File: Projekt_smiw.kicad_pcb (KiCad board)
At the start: 4 copper layers, 66.9 x 38.2 mm, 24 parts, among them J1 USB_C_Receptacle_USB2.0, J4 Conn_02x12_Odd_Even, J5 Conn_02x12_Odd_Even, SW1 SW_Omron_B3FS, SW2 SW_Omron_B3FS, U1 USBLC6-2P6, U2 NCP1117-3.3_SOT223, U4 ESP32-S3-PICO-1

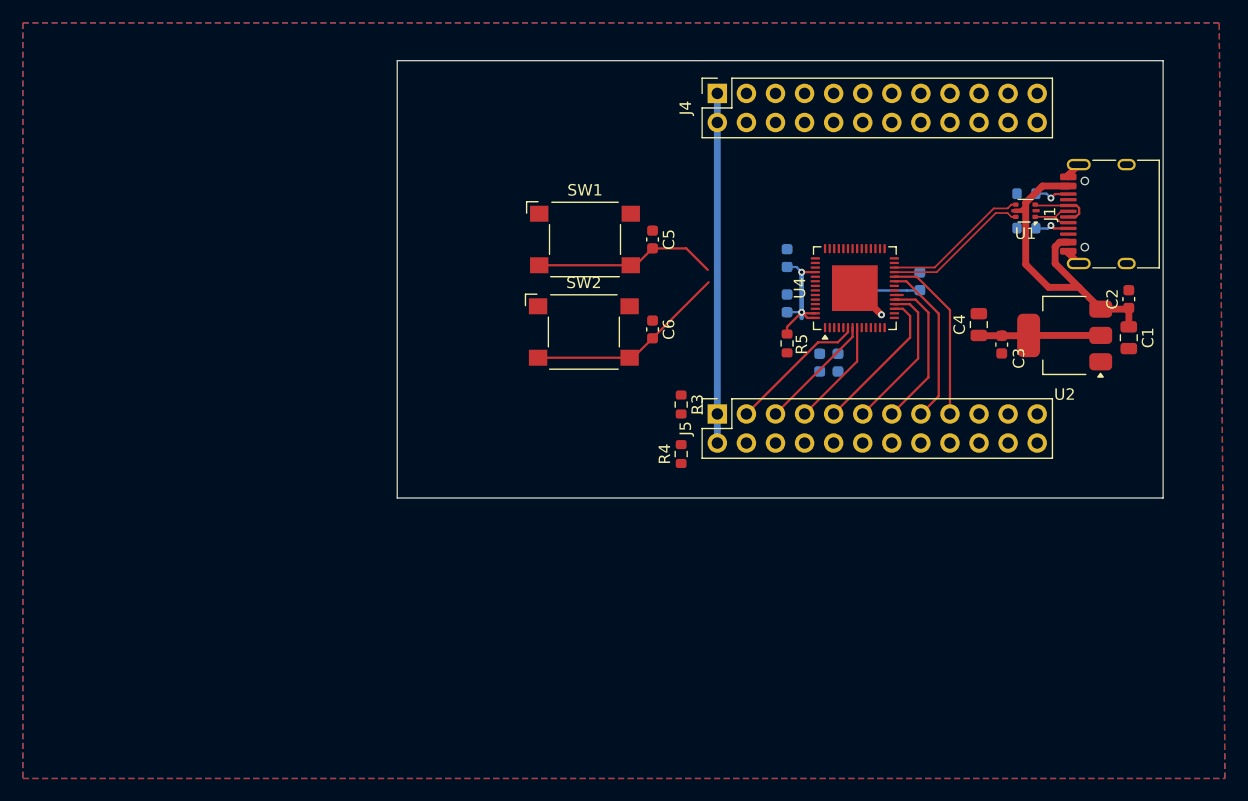
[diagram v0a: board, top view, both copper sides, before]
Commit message: zegar tesz
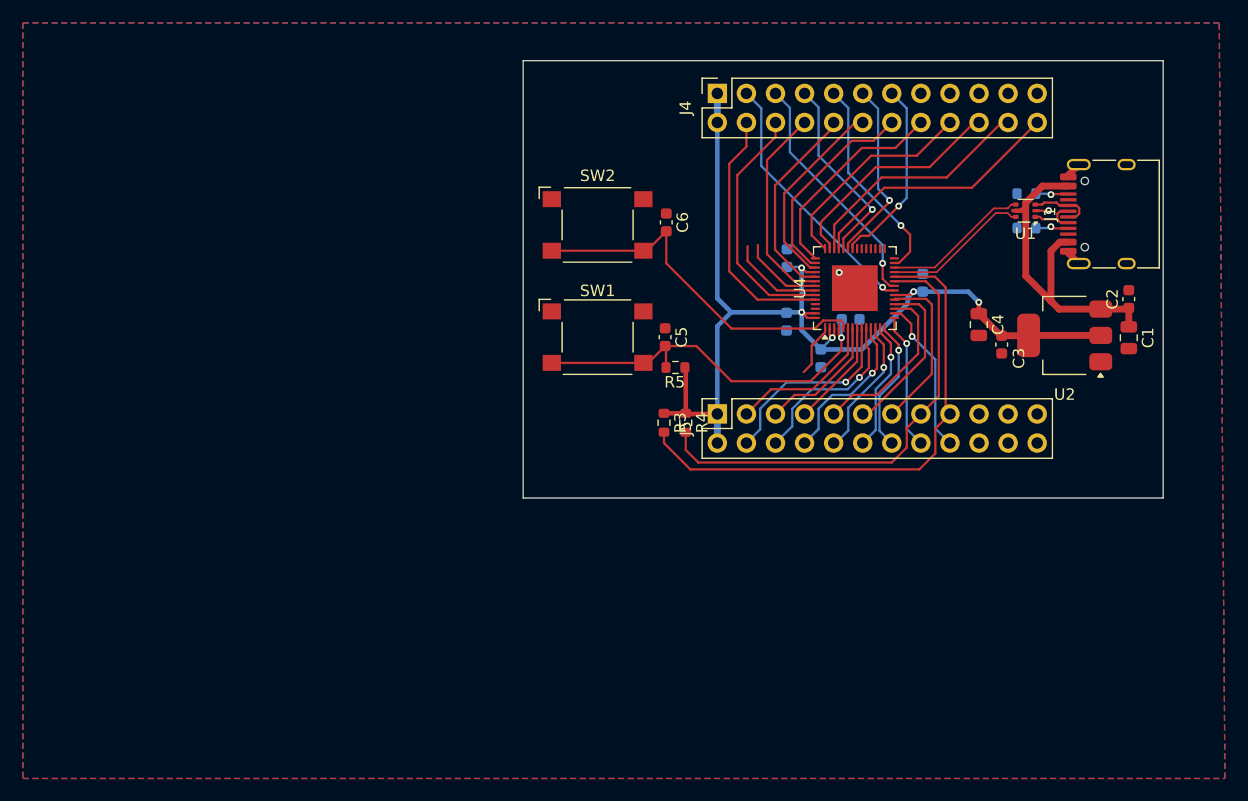
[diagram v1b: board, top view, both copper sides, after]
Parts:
- moved R5 9.97 mm to (186.0, 64.6), turned to 180 degrees
- moved C6 9.43 mm to (185.2, 51.9)
- moved SW2 9.43 mm to (179.2, 52.1)
- moved C5 8.60 mm to (185.1, 62.0)
- moved SW1 8.60 mm to (179.2, 62.0)
- moved C7 3.93 mm to (201.3, 60.4), turned to 180 degrees
- moved R4 2.76 mm to (186.9, 69.4), turned to -90 degrees
- moved R3 2.19 mm to (185.0, 69.4)
- moved C9 1.60 mm to (195.7, 60.6), turned to -90 degrees
- moved C10 0.39 mm to (198.7, 63.8)
- moved C11 0.28 mm to (207.6, 57.2)
- turned C4 to -90 degrees
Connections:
- J4 pad 10: /GPIO33 -> /MTDI
- J4 pad 12: /GPIO34 -> /MTDO
- J4 pad 14: /GPIO35 -> /MTCK
- J4 pad 16: /GPIO36 -> /GPIO38
- J4 pad 20: /GPIO38 -> /GPIO36
- J4 pad 22: /GPIO45 -> /GPIO35
- J4 pad 24: /GPIO46 -> /GPIO34
- J4 pad 3: /MTCK -> /XTAL_32K_P
- J4 pad 4: /MTDO -> /GPIO46
- J4 pad 5: /GPIO21 -> /XTAL_32K_N
- J4 pad 6: /MTDI -> /GPIO45
- J4 pad 7: /XTAL_32K_P -> /GPIO33
- J4 pad 9: /XTAL_32K_N -> /GPIO21
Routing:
- net +3.3V: track 59.4 -> 93.8 mm, vias 2 -> 5
- net /SCL: track 15.5 -> 46.6 mm
- net /SDA: track 14.6 -> 40.9 mm
- net /XTAL_32K_P: track 0.00 -> 23.2 mm, vias 0 -> 1
- net /GPIO34: track 0.00 -> 22.7 mm
- net /GPIO46: track 0.00 -> 22.2 mm
- net /GPIO45: track 0.00 -> 21.7 mm
- net /XTAL_32K_N: track 0.00 -> 21.3 mm, vias 0 -> 1
- net /GPIO35: track 0.00 -> 21.0 mm
- net /GPIO36: track 0.00 -> 20.1 mm
- net /GPIO37: track 0.00 -> 18.8 mm
- net /GPIO38: track 0.00 -> 18.5 mm
- net /GPIO21: track 0.00 -> 18.4 mm, vias 0 -> 1
- net /MTMS: track 0.00 -> 18.1 mm
- net /MTCK: track 0.00 -> 18.1 mm
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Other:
- board size 66.9 x 38.2 mm -> 55.9 x 38.2 mm
